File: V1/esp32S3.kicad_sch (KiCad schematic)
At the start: 19 parts, among them Q1 BC817-25Q-7-F, Q2 BC817-25Q-7-F, SW1 KH-6X6X5H-STM, SW2 KH-6X6X5H-STM, U4 ESP32-S3-WROOM-1(N8R2), U5 YTC-TC16S-24, U6 CP2102N-A02-GQFN28R

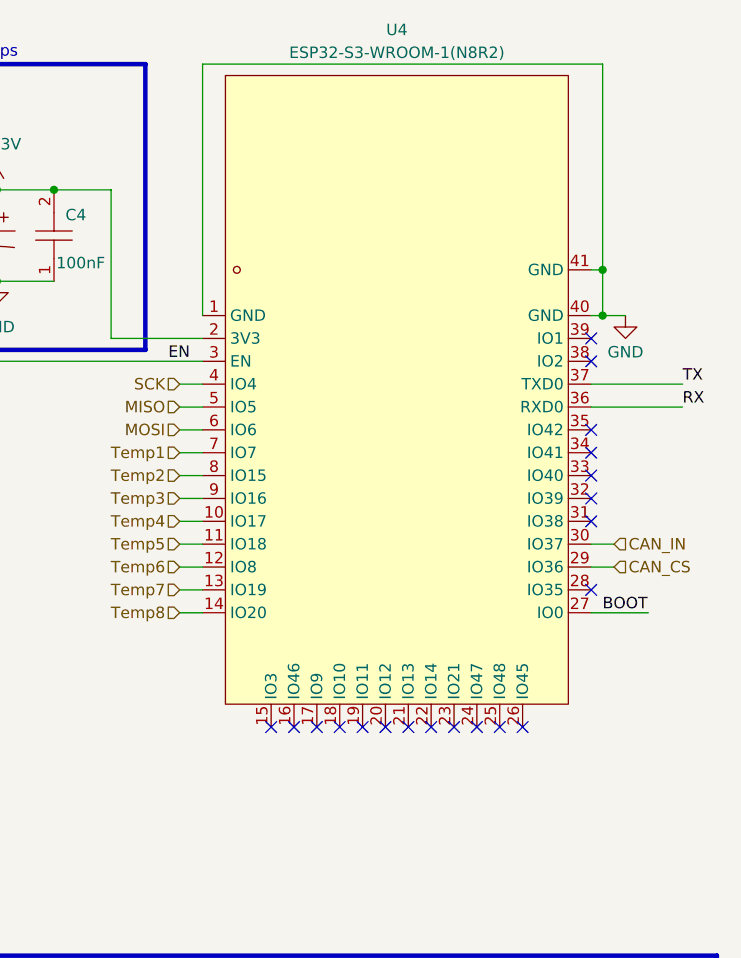
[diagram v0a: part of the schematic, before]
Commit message: Latest
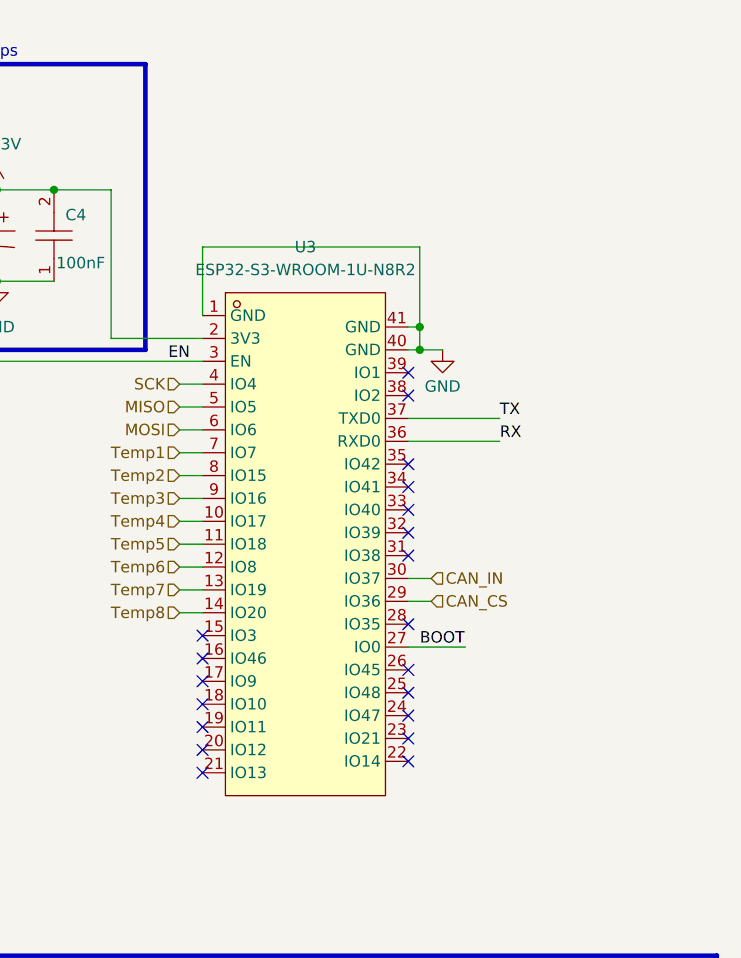
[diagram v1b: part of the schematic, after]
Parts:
- removed U4: ESP32-S3-WROOM-1(N8R2), easyeda2kicad:WIRELM-SMD_ESP32-S3-WROOM-1, symbol easyeda2kicad:ESP32-S3-WROOM-1(N8R2)
- added U3: ESP32-S3-WROOM-1U-N8R2, easyeda2kicad:WIRELM-SMD_ESP32-S3-WROOM-1U, symbol easyeda2kicad:ESP32-S3-WROOM-1U-N8R2
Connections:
- net +3.3V: now also U3.2 (3V3)
- net BOOT: now also U3.27 (IO0)
- net CAN_CS: now also U3.29 (IO36)
- net CAN_IN: now also U3.30 (IO37)
- net EN: now also U3.3 (EN)
- net GND: now also U3.1 (GND), U3.40 (GND), U3.41 (GND)
- net MISO: now also U3.5 (IO5)
- net MOSI: now also U3.6 (IO6)
- net RX: now also U3.36 (RXD0)
- net SCK: now also U3.4 (IO4)
- net TX: now also U3.37 (TXD0)
- net Temp1: now also U3.7 (IO7)
- net Temp2: now also U3.8 (IO15)
- net Temp3: now also U3.9 (IO16)
- net Temp4: now also U3.10 (IO17)
- net Temp5: now also U3.11 (IO18)
- net Temp6: now also U3.12 (IO8)
- net Temp7: now also U3.13 (IO19)
- net Temp8: now also U3.14 (IO20)
